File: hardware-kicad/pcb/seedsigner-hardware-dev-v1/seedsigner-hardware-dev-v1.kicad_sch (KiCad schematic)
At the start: 6 parts, among them J1 Conn_01x08_MountingPin

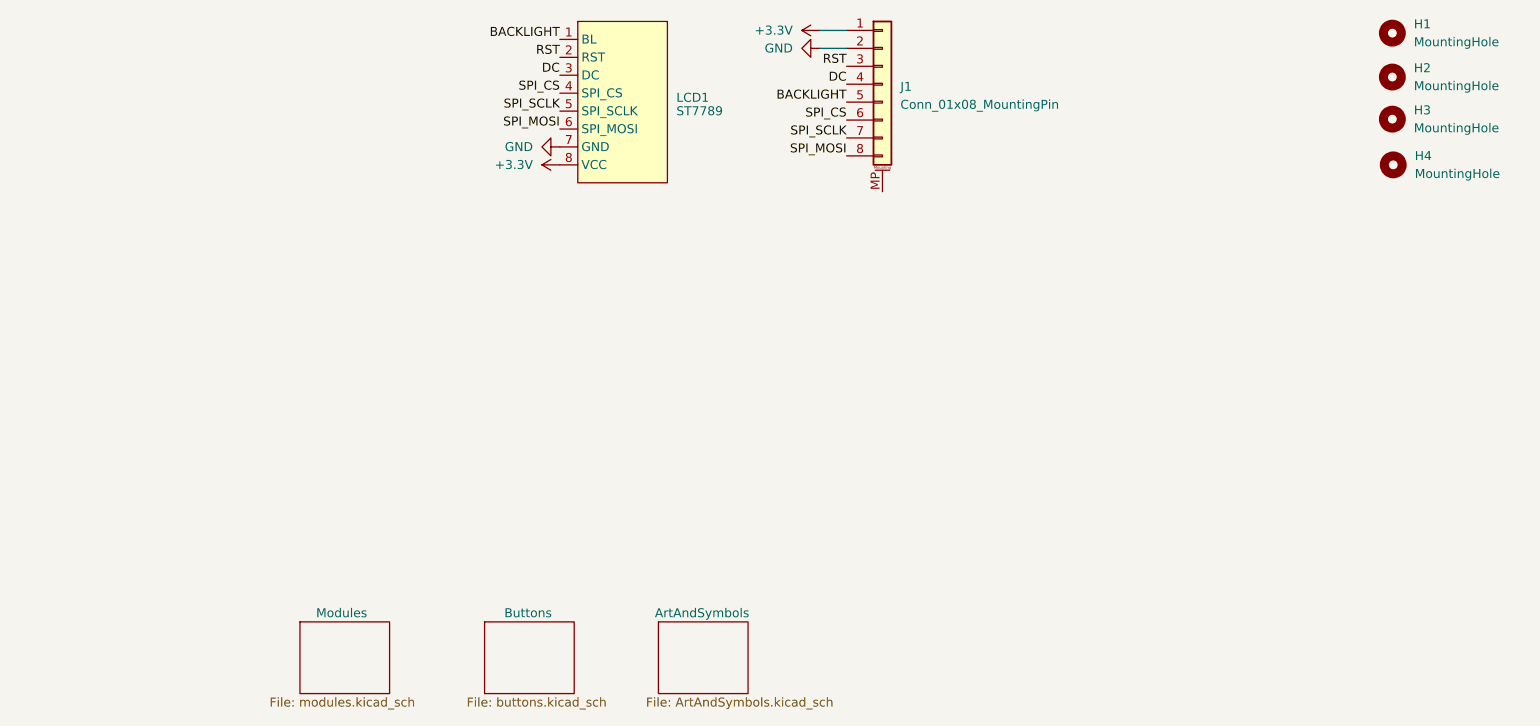
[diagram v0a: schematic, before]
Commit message: 2 different pcbs almost done
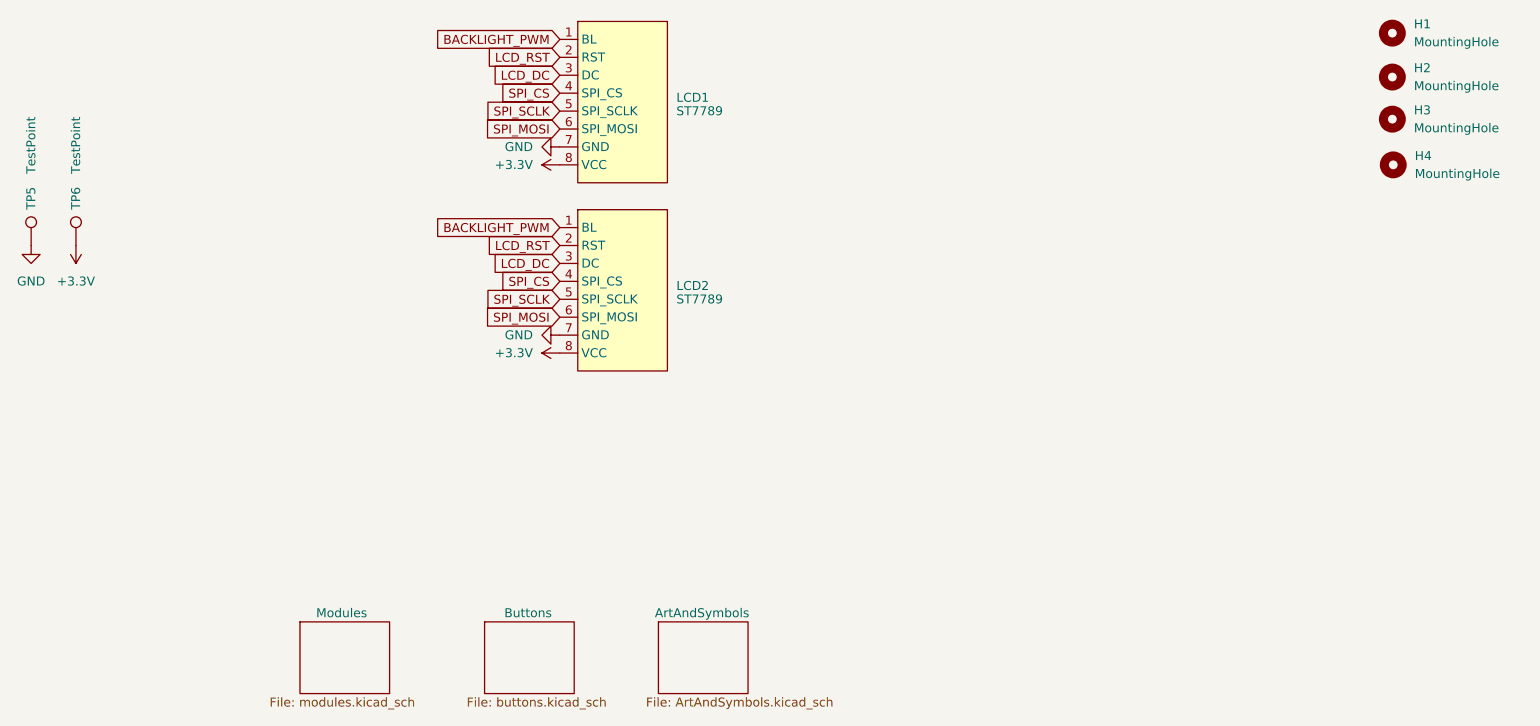
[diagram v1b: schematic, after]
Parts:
- removed J1: Conn_01x08_MountingPin, Connector_PinHeader_2.54mm:PinHeader_1x08_P2.54mm_Horizontal, symbol Connector_Generic_MountingPin:Conn_01x08_MountingPin
- added LCD2: ST7789, Connector_PinHeader_2.54mm:PinHeader_1x08_P2.54mm_Vertical, symbol SeedSigner:LCD_ST7789
- added TP5, TP6: TestPoint, TestPoint:TestPoint_Pad_D1.0mm, symbol Connector:TestPoint
- H1, H2, H3, H4: now left out of the parts list
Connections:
- net +3.3V: now also LCD2.8 (VCC), TP6.1
- net GND: now also LCD2.7 (GND), TP5.1
- net SPI_CS: now also LCD2.4 (SPI_CS)
- net SPI_MOSI: now also LCD2.6 (SPI_MOSI)
- net SPI_SCLK: now also LCD2.5 (SPI_SCLK)
- net BACKLIGHT renamed BACKLIGHT_PWM
- net BACKLIGHT_PWM: now also LCD2.1 (BL)
- net DC renamed LCD_DC
- net LCD_DC: now also LCD2.3 (DC)
- net RST renamed LCD_RST
- net LCD_RST: now also LCD2.2 (RST)
